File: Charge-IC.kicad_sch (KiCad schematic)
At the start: 35 parts

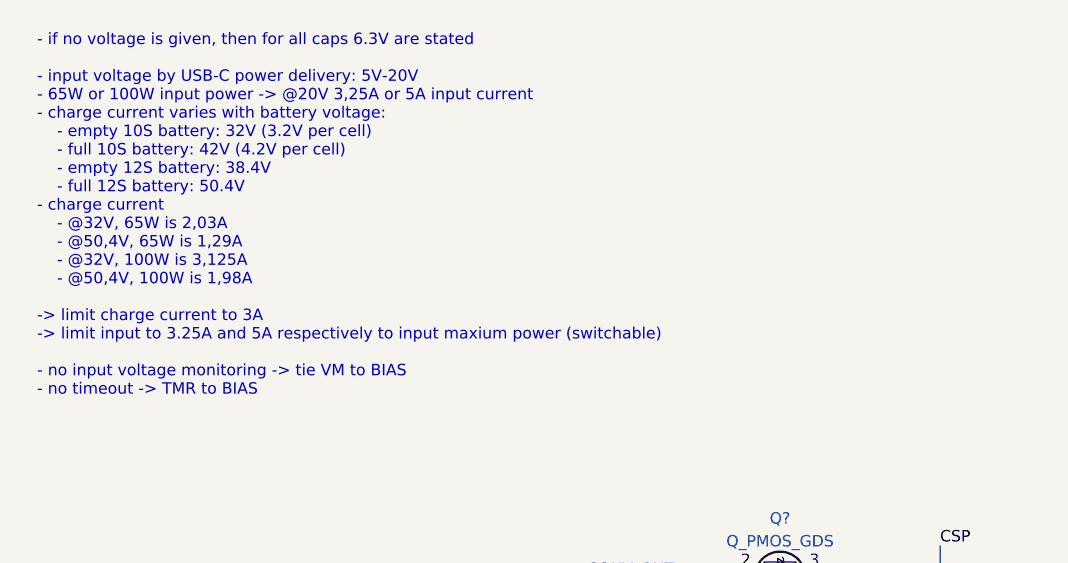
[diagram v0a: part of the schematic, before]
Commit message: Finish boost converter
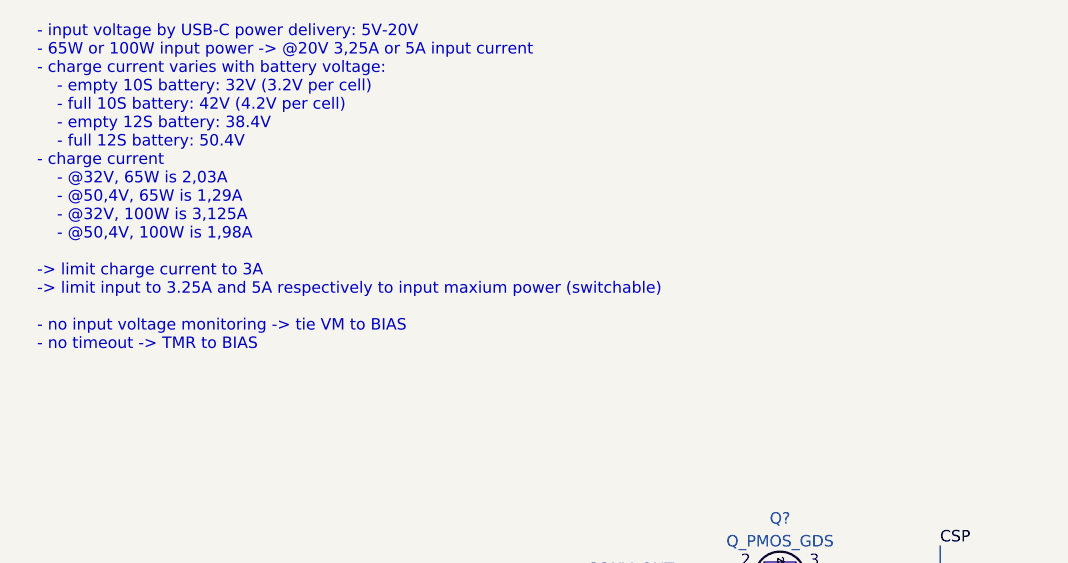
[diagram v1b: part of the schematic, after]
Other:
- note added: "- input voltage by USB-C power delivery: 5V-20V - 65W or 100W input power -> @20V 3,25A or 5A input current - charge current varies with battery voltage: - empty 10S battery: 32V (3.2V per cell) - full 10S battery: 42V (4.2V per cell) - empty 12S battery: 38.4V - full 12S battery: 50.4V - charge current - @32V, 65W is 2,03A - @50,4V, 65W is 1,29A - @32V, 100W is 3,125A - @50,4V, 100W is 1,98A -> 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"
- note removed: "- if no voltage is given, then for all caps 6.3V are stated - input voltage by USB-C power delivery: 5V-20V - 65W or 100W input power -> @20V 3,25A or 5A input current - charge current varies with battery voltage: - empty 10S battery: 32V (3.2V per cell) - full 10S battery: 42V (4.2V per cell) - empty 12S battery: 38.4V - full 12S battery: 50.4V - charge current - @32V, 65W is 2,03A - @50,4V, 65W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"
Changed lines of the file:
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@@
     (effects (font (size 1.27 1.27)) (justify left bottom))
   )
-  (text "- if no voltage is given, then for all caps 6.3V are stated\n\n- input voltage by USB-C power delivery: 5V-20V\n- 65W or 100W input power -> @20V 3,25A or 5A input current\n- charge current varies with battery voltage:\n	- empty 10S battery: 32V (3.2V per cell)\n	- full 10S battery: 42V (4.2V per cell)\n	- empty 12S battery: 38.4V\n	- full 12S battery: 50.4V\n- charge current \n	- @32V, 65W is 2,03A\n	- @50,4V, 65W is 1,29A\n	- @32V, 100W is 3,125A\n	- @50,4V, 100W is 1,98A\n\n-> limit charge current to 3A\n-> limit input to 3.25A and 5A respectively to input maxium power (switchable)\n\n- no input voltage monitoring -> tie VM to BIAS\n- no timeout -> TMR to BIAS"
-    (at 13.97 55.88 0)
+  (text "- input voltage by USB-C power delivery: 5V-20V\n- 65W or 100W input power -> @20V 3,25A or 5A input current\n- charge current varies with battery voltage:\n	- empty 10S battery: 32V (3.2V per cell)\n	- full 10S battery: 42V (4.2V per cell)\n	- empty 12S battery: 38.4V\n	- full 12S battery: 50.4V\n- charge current \n	- @32V, 65W is 2,03A\n	- @50,4V, 65W is 1,29A\n	- @32V, 100W is 3,125A\n	- @50,4V, 100W is 1,98A\n\n-> limit charge current to 3A\n-> limit input to 3.25A and 5A respectively to input maxium power (switchable)\n\n- no input voltage monitoring -> tie VM to BIAS\n- no timeout -> TMR to BIAS"
+    (at 13.97 50.8 0)
     (effects (font (size 1.27 1.27)) (justify left bottom))
   )
